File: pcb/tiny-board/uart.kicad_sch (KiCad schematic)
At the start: 14 parts, among them J3 Serial, J6 UART1, U8 W65C51NxP, U9 MAX232, Y1 1.8432 MHz

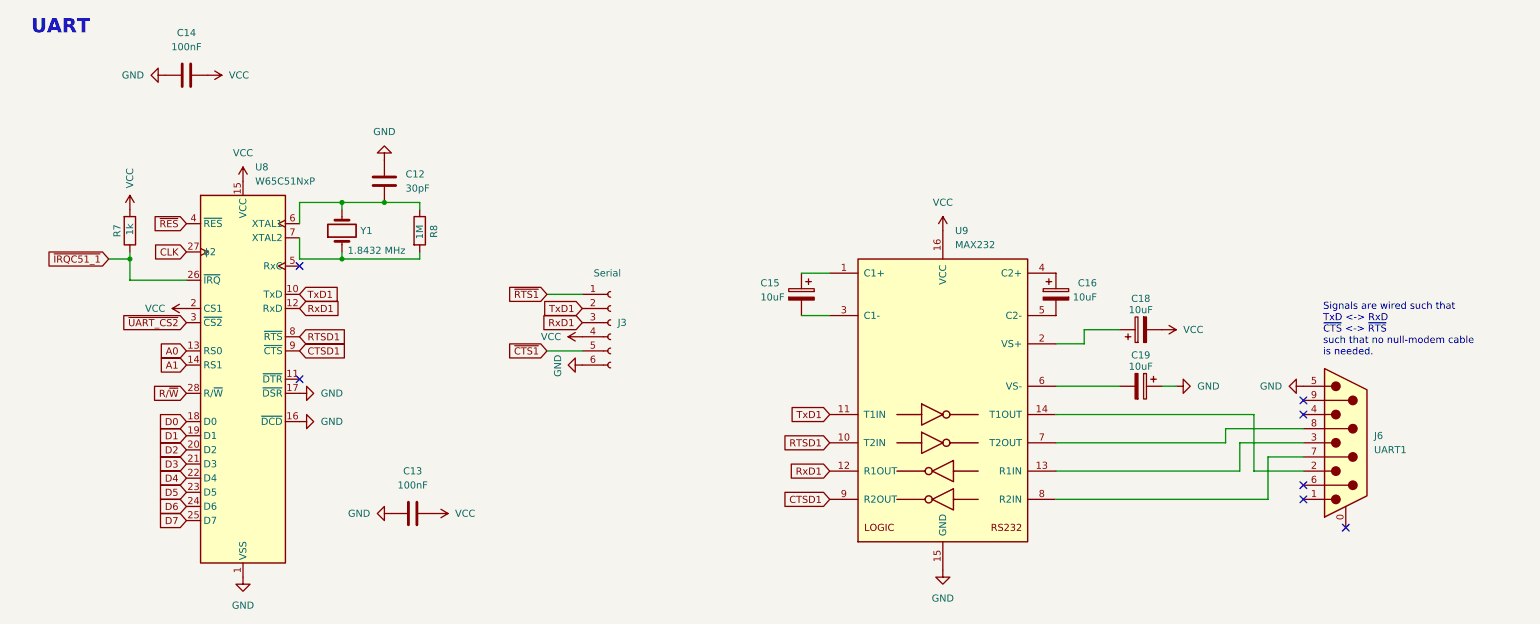
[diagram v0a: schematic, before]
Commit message: Saving tiny board design
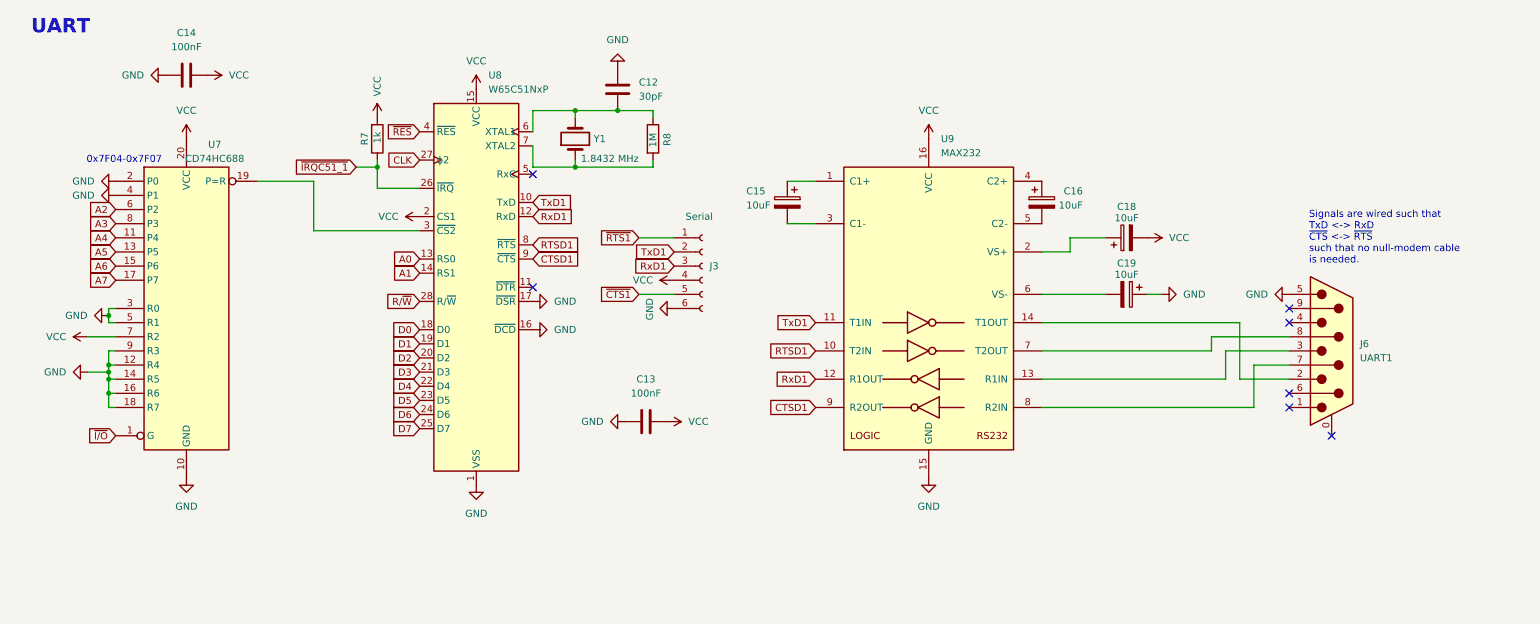
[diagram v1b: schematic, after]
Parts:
- added U7: CD74HC688, Package_DIP:DIP-20_W7.62mm_Socket, symbol 74xx:74HC688
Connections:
- net GND: now also U7.10 (GND), U7.12 (R4), U7.14 (R5), U7.16 (R6), U7.18 (R7), U7.2 (P0), U7.3 (R0), U7.4 (P1), U7.5 (R1), U7.9 (R3)
- net VCC: now also U7.20 (VCC), U7.7 (R2)
- net ~{UART_CS2}: no longer names the net of U8.3 (~{CS2})
- net ~{UART_CS2}: now also U7.19 (P=R)
- new net A2: U7.6 (P2)
- new net A3: U7.8 (P3)
- new net A4: U7.11 (P4)
- new net A5: U7.13 (P5)
- new net A6: U7.15 (P6)
- new net A7: U7.17 (P7)
- new net ~{I/O}: U7.1 (G)
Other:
- note added: "0x7F04-0x7F07"
- moved on the sheet: C12, C13, C15, C16, C18, C19, J3, J6, R7, R8, U8, U9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
